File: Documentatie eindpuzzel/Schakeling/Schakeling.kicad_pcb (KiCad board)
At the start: 2 copper layers, 65.5 x 78.5 mm, 33 parts, among them Q1 BC817, Q2 BC817

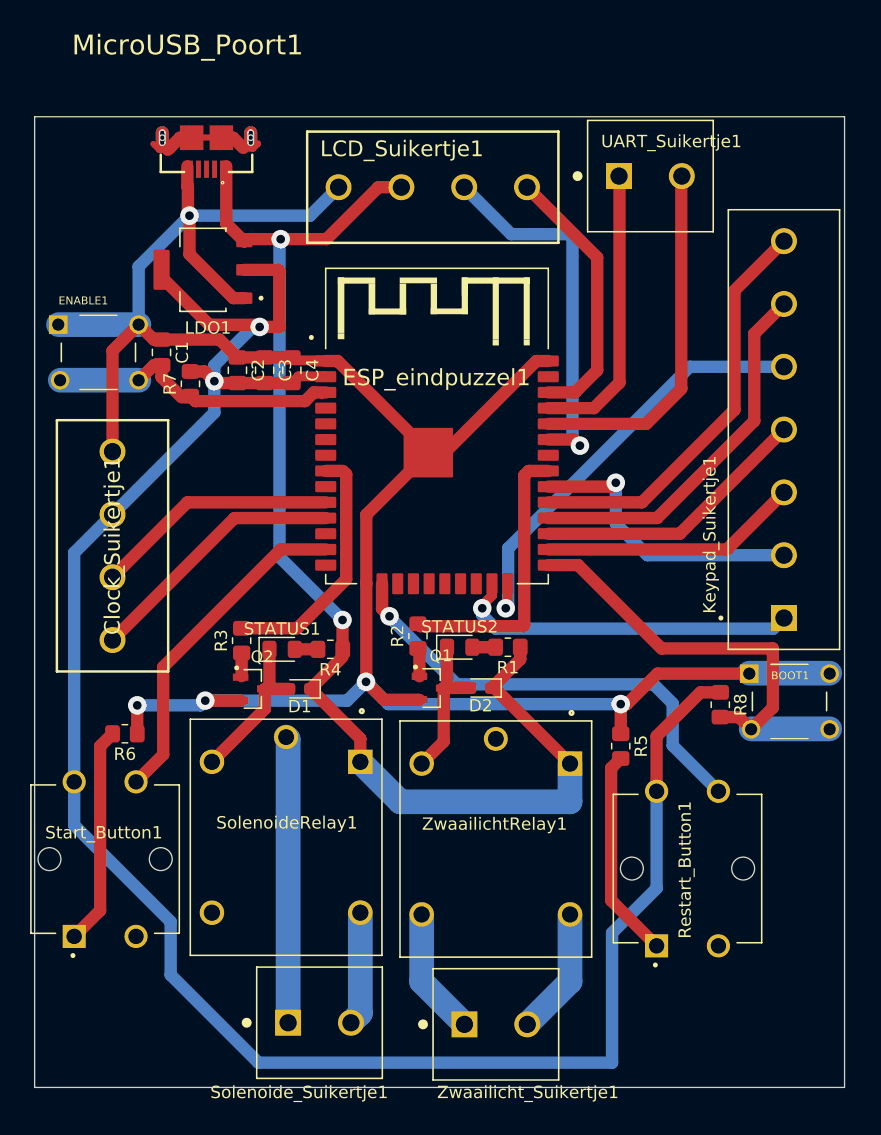
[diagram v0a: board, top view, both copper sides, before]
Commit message: Updates pcb eindpuzzel
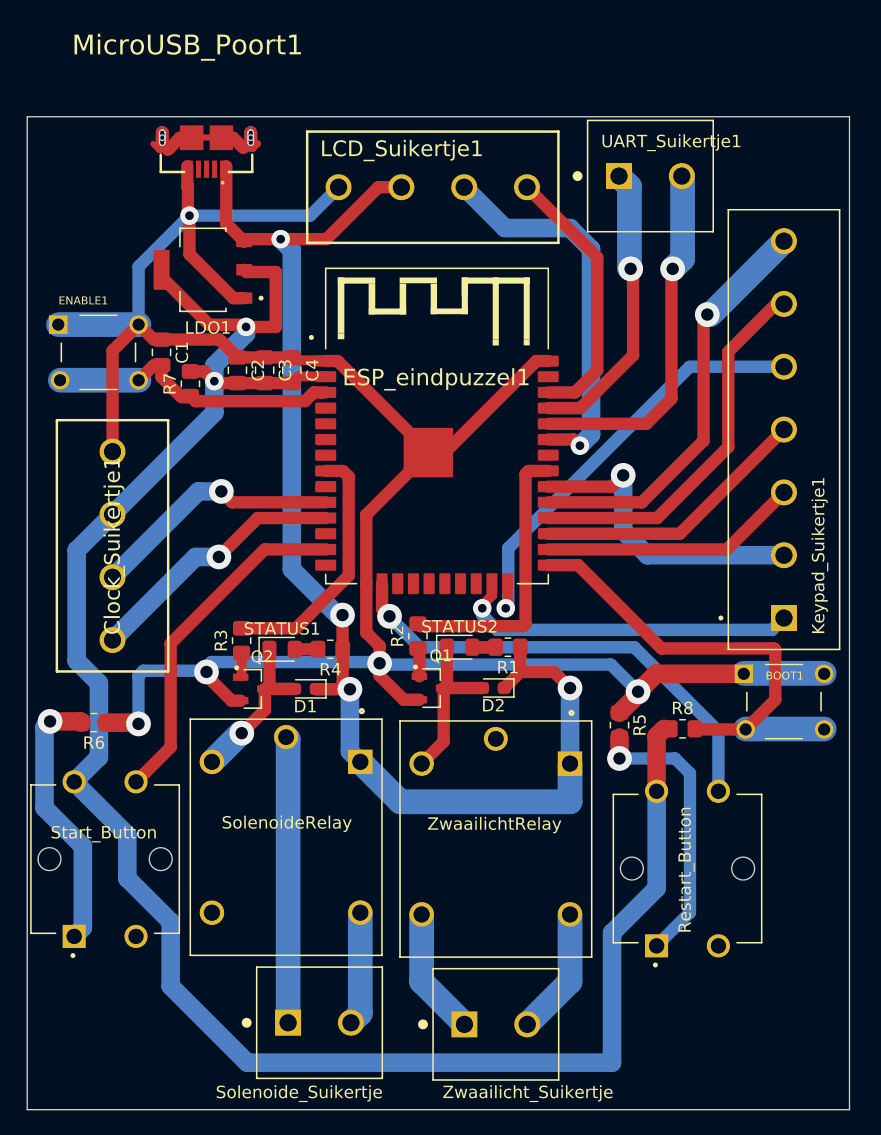
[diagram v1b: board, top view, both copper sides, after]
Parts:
- moved R8 3.62 mm to (111.3, 81.6), turned to 0 degrees
- moved R6 2.66 mm to (63.7, 81.1)
- moved R5 1.70 mm to (106.2, 81.3)
- moved D2 1.03 mm to (96.0, 78.3)
- moved D1 0.46 mm to (80.8, 78.4)
- moved BOOT1 0.45 mm to (119.5, 79.4)
- renumbered Restart_Button1 to Restart_Button, SolenoideRelay1 to SolenoideRelay, Solenoide_Suikertje1 to Solenoide_Suikertje, Start_Button1 to Start_Button, ZwaailichtRelay1 to ZwaailichtRelay, Zwaailicht_Suikertje1 to Zwaailicht_Suikertje
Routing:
- net Net-(R5-Pad2): track 17.0 -> 23.0 mm, vias 0 -> 1
- net GND: track 188.3 -> 194.0 mm
- net 3.3V: track 166.1 -> 160.8 mm
- net Net-(R6-Pad2): track 17.7 -> 21.9 mm, vias 0 -> 1
- net 5V: track 102.9 -> 105.6 mm, vias 2 -> 4
- net Net-(BOOT1-Pad3): track 37.5 -> 39.2 mm
- net IO18: track 23.6 -> 24.8 mm
- net Net-(D2-Pad2): track 12.4 -> 13.4 mm
- net IO21: track 30.4 -> 31.4 mm
- net IO13: track 37.4 -> 38.2 mm
- net IO14: track 27.3 -> 28.0 mm
- net IO25: track 19.7 -> 20.5 mm, vias 0 -> 1
- net Net-(D1-Pad2): track 13.0 -> 13.6 mm, vias 0 -> 1
- net IO5: track 33.5 -> 34.0 mm, vias 0 -> 1
- net Net-(ESP_eindpuzzel1-Pad35): track 23.3 -> 23.6 mm, vias 0 -> 1
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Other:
- board size 65.5 x 78.5 mm -> 66.5 x 80.3 mm

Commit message: Veel nieuwe aanpassing in de Kicad files ( en ook een paar in de code)
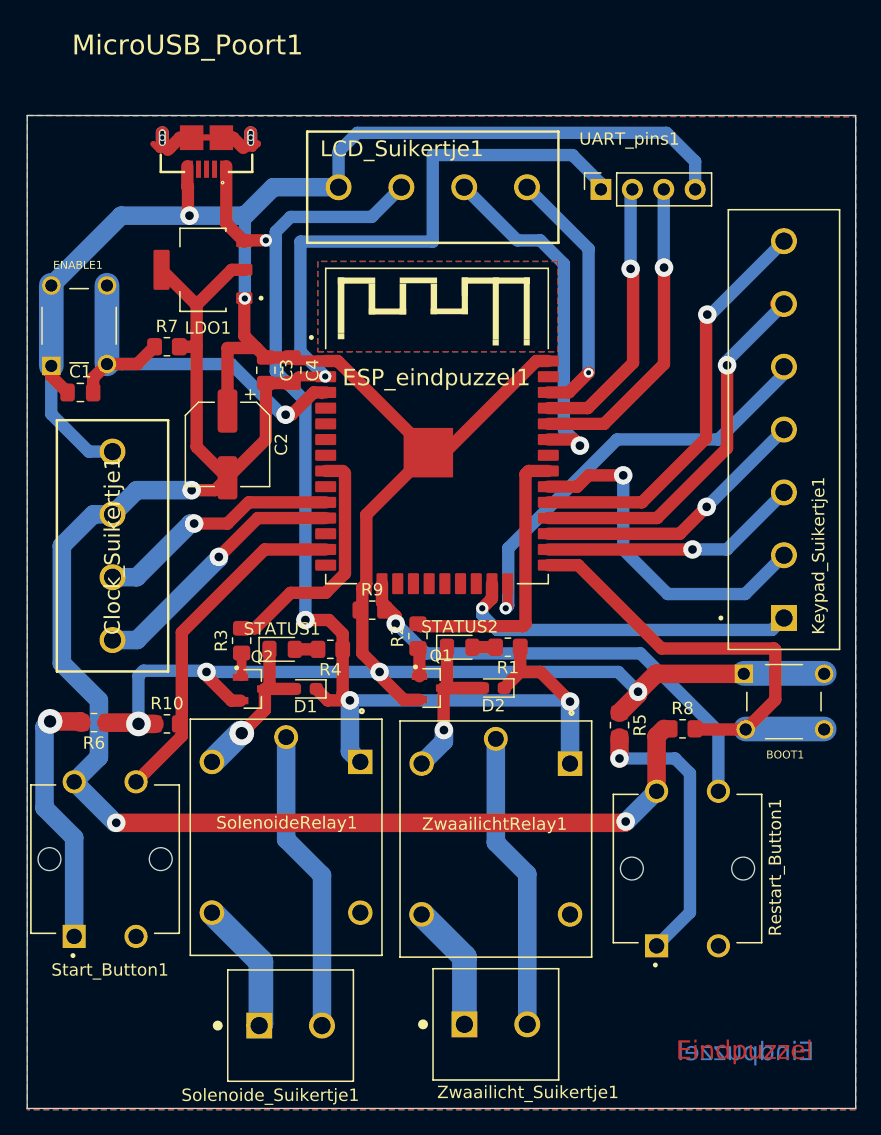
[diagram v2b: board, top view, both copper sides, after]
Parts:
- removed UART_Suikertje1: 282841-2, components:TE_282841-2
- added R10: 1k, Resistor_SMD:R_0805_2012Metric_Pad1.20x1.40mm_HandSolder, F.Cu at (69.6, 81.2)
- added R9: 1k, Resistor_SMD:R_0805_2012Metric_Pad1.20x1.40mm_HandSolder, F.Cu at (86.2, 72.0)
- added UART_pins1: Conn_01x04_Female, Connector_PinSocket_2.54mm:PinSocket_1x04_P2.54mm_Vertical, F.Cu at (104.7, 38.0)
- C2: footprint Capacitor_SMD:C_0805_2012Metric_Pad1.18x1.45mm_HandSolder -> Capacitor_SMD:CP_Elec_6.3x7.7
- moved C1 7.32 mm to (62.6, 54.4), turned to 0 degrees
- moved C2 6.05 mm to (74.5, 58.6)
- moved R7 3.55 mm to (69.6, 50.7), turned to 0 degrees
- moved ENABLE1 2.66 mm to (62.5, 49.0), turned to 90 degrees
- moved Solenoide_Suikertje1 2.35 mm to (79.6, 105.6)
- moved C3 0.10 mm to (77.6, 52.6)
- renumbered Restart_Button to Restart_Button1, SolenoideRelay to SolenoideRelay1, Solenoide_Suikertje to Solenoide_Suikertje1, Start_Button to Start_Button1, ZwaailichtRelay to ZwaailichtRelay1, Zwaailicht_Suikertje to Zwaailicht_Suikertje1
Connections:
- ESP_eindpuzzel1 pad 34: Net-(ESP_eindpuzzel1-Pad34) -> RX
- ESP_eindpuzzel1 pad 35: Net-(ESP_eindpuzzel1-Pad35) -> TX
- SolenoideRelay1 pad NC: Net-(SolenoideRelay1-PadNC) -> unconnected-(SolenoideRelay1-PadNC)
- SolenoideRelay1 pad NO: unconnected-(SolenoideRelay1-PadNO) -> Net-(SolenoideRelay1-PadNO)
- Solenoide_Suikertje1 pad 1: Net-(SolenoideRelay1-PadCOM) -> Net-(SolenoideRelay1-PadNO)
- Solenoide_Suikertje1 pad 2: Net-(SolenoideRelay1-PadNC) -> Net-(SolenoideRelay1-PadCOM)
- ZwaailichtRelay1 pad COM: unconnected-(ZwaailichtRelay1-PadCOM) -> Net-(ZwaailichtRelay1-PadCOM)
- ZwaailichtRelay1 pad NC: Net-(ZwaailichtRelay1-PadNC) -> unconnected-(ZwaailichtRelay1-PadNC)
- Zwaailicht_Suikertje1 pad 2: Net-(ZwaailichtRelay1-PadNC) -> Net-(ZwaailichtRelay1-PadCOM)
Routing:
- net GND: track 194.0 -> 234.0 mm, vias 5 -> 6
- net Net-(ESP_eindpuzzel1-Pad34): track 29.2 -> 0.00 mm, vias 1 -> 0
- net RX: track 0.00 -> 25.5 mm, vias 0 -> 1
- net Net-(ZwaailichtRelay1-PadCOM): track 0.00 -> 24.1 mm
- net Net-(ESP_eindpuzzel1-Pad35): track 23.6 -> 0.00 mm, vias 1 -> 0
- net TX: track 0.00 -> 22.5 mm, vias 0 -> 1
- net 3.3V: track 160.8 -> 176.4 mm, vias 2 -> 4
- net Net-(SolenoideRelay1-PadNO): track 0.00 -> 10.8 mm
- net Net-(ZwaailichtRelay1-PadNC): track 10.3 -> 0.00 mm
- net Net-(C1-Pad2): track 23.8 -> 34.1 mm, vias 0 -> 1
- net Net-(SolenoideRelay1-PadNC): track 9.21 -> 0.00 mm
- net IO18: track 24.8 -> 28.2 mm
- net IO21: track 31.4 -> 28.6 mm
- net 5V: track 105.6 -> 103.2 mm
- net Net-(SolenoideRelay1-PadCOM): track 23.2 -> 24.5 mm
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- added copper zone on B.Cu, net GND
- added copper zone on F.Cu, net GND
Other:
- board size 66.5 x 80.3 mm -> 67 x 80.3 mm
- board text added: "Eindpuzzel"
